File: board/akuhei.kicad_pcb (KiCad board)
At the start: 2 copper layers, 23 x 23.4 mm, 9 parts, among them J1 CLOCKPORT, J2 I2C, U2 PCA9564, U3 TLV70233DBV

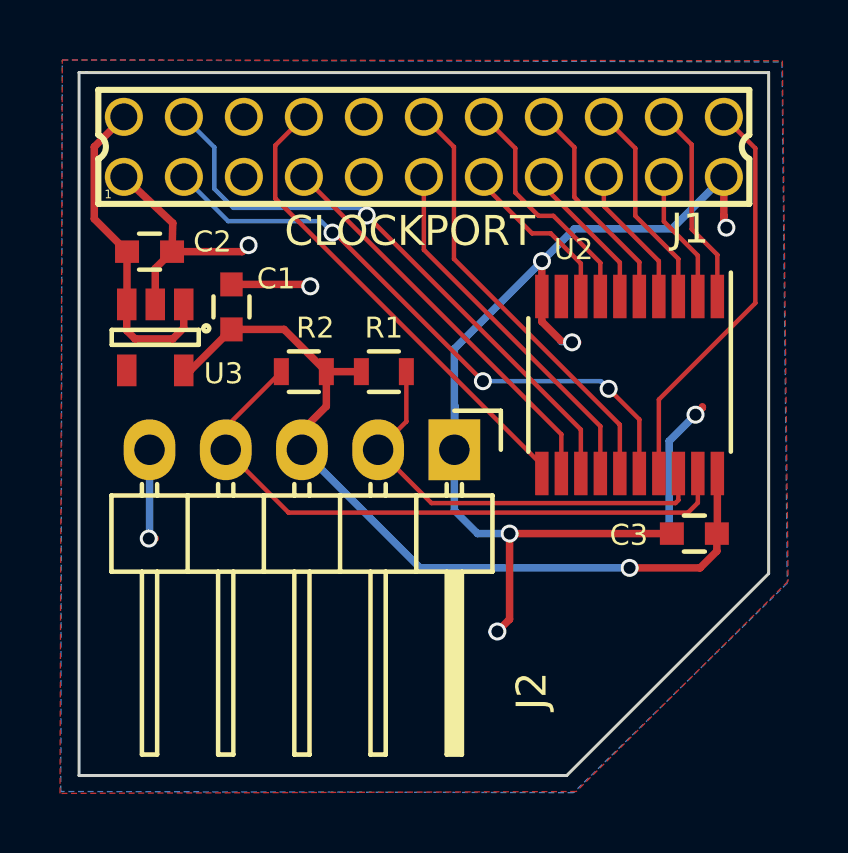
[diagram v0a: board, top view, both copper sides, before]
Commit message: removing error
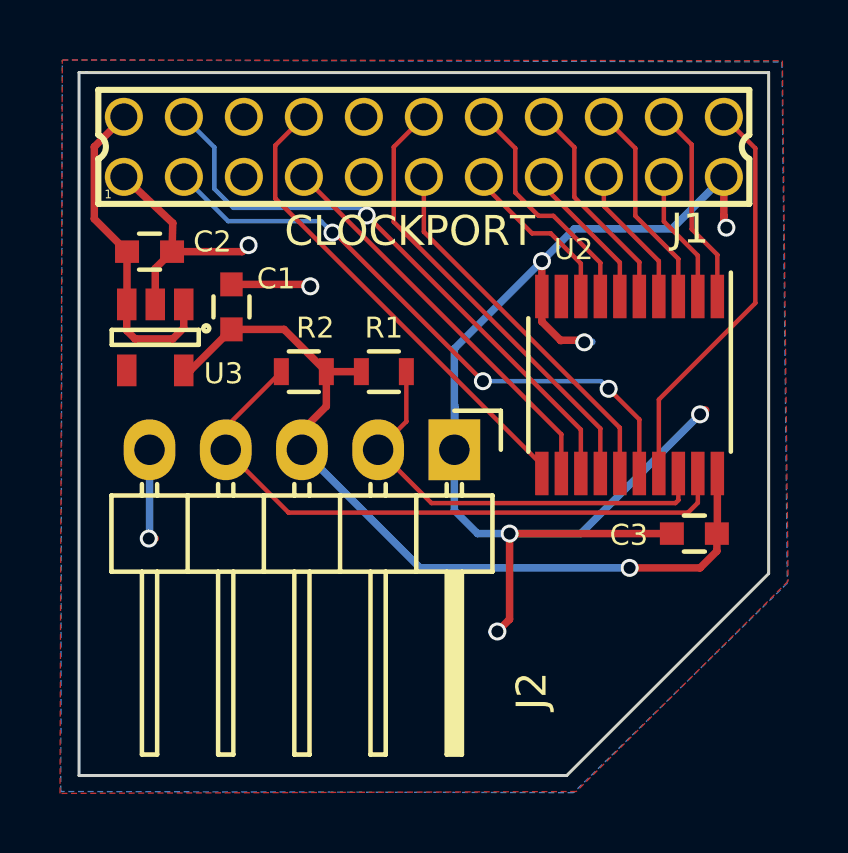
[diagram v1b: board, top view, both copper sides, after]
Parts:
- C1: value 1u -> 1uF
- C2: value u1 -> 0.1uF
- R1, R2: value 4k7 -> 4.7k
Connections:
- J1 pad 11: /A1 -> /A2
- J1 pad 12: /A2 -> /A1
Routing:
- net GND: track 48.9 -> 58.2 mm, vias 7 -> 9
- net (no net): track 5.22 -> 0.00 mm, vias 2 -> 0
- net /A1: track 12.3 -> 15.2 mm
- net /A2: track 14.6 -> 12.6 mm
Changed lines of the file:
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@@
     (links 36)
     (no_connects 0)
-    (area 132.3867 96.2279 160.286701 124.42)
+    (area 136.601999 96.596999 159.689001 120.128501)
     (thickness 1.6)
     (drawings 9)
-    (tracks 163)
+    (tracks 165)
     (zones 0)
     (modules 9)
@@
     (visible_elements 7FFFFFFF)
     (pcbplotparams
-      (layerselection 0x20020_00000000)
+      (layerselection 0x210f8_80000001)
       (usegerberextensions false)
       (excludeedgelayer true)
@@
       (viasonmask false)
       (mode 1)
-      (useauxorigin false)
+      (useauxorigin true)
       (hpglpennumber 1)
       (hpglpenspeed 20)
@@
       (effects (font (size 0.7 0.7) (thickness 0.15)))
     )
-    (fp_text value 1u (at -0.0381 0.0127 180) (layer F.Fab)
+    (fp_text value 1uF (at -0.0381 0.0127 180) (layer F.Fab)
       (effects (font (size 0.5 0.5) (thickness 0.125)))
     )
@@
       (effects (font (size 0.7 0.7) (thickness 0.15)))
     )
-    (fp_text value u1 (at 0.0254 -0.0508 90) (layer F.Fab)
+    (fp_text value 0.1uF (at 0.0254 -0.0508 90) (layer F.Fab)
       (effects (font (size 0.5 0.5) (thickness 0.125)))
     )
@@
       (net 11 "Net-(J1-Pad10)"))
     (pad 11 thru_hole circle (at 0 1) (size 1.27 1.27) (drill 0.9) (layers *.Cu *.Mask)
+      (net 13 /A2))
+    (pad 12 thru_hole circle (at 0 -1) (size 1.27 1.27) (drill 0.9) (layers *.Cu *.Mask)
       (net 12 /A1))
-    (pad 12 thru_hole circle (at 0 -1) (size 1.27 1.27) (drill 0.9) (layers *.Cu *.Mask)
-      (net 13 /A2))
     (pad 13 thru_hole circle (at 2 1) (size 1.27 1.27) (drill 0.9) (layers *.Cu *.Mask)
       (net 14 /D7))
@@
       (effects (font (size 0.7 0.7) (thickness 0.15)))
     )
-    (fp_text value 4k7 (at -0.0381 0 270) (layer F.Fab)
+    (fp_text value 4.7k (at -0.0381 0 270) (layer F.Fab)
       (effects (font (size 0.5 0.5) (thickness 0.125)))
     )
@@
       (effects (font (size 0.7 0.7) (thickness 0.15)))
     )
-    (fp_text value 4k7 (at 0.0254 -0.0254 90) (layer F.Fab)
+    (fp_text value 4.7k (at 0.0254 -0.0254 90) (layer F.Fab)
       (effects (font (size 0.5 0.5) (thickness 0.125)))
     )
@@
   (gr_line (start 159.639 96.647) (end 159.639 113.3475) (angle 90) (layer Edge.Cuts) (width 0.1))
   (gr_line (start 136.906 96.647) (end 159.639 96.647) (angle 90) (layer Edge.Cuts) (width 0.1))
-  (segment (start 156.3243 111.9759) (end 156.3243 108.9279) (width 0.25) (layer B.Cu) (net 0))
-  (segment (start 157.4292 107.823) (end 157.4292 107.7849) (width 0.25) (layer F.Cu) (net 0))
-  (segment (start 157.2006 108.0516) (end 157.4292 107.823) (width 0.25) (layer F.Cu) (net 0))
-  (via (at 157.2006 108.0516) (size 0.6) (drill 0.4) (layers F.Cu B.Cu) (net 0))
-  (segment (start 156.3243 108.9279) (end 157.2006 108.0516) (width 0.25) (layer B.Cu) (net 0))
-  (segment (start 152.7175 105.6132) (end 153.0604 105.6132) (width 0.25) (layer B.Cu) (net 0))
-  (segment (start 153.0858 105.6386) (end 153.2763 105.6386) (width 0.25) (layer F.Cu) (net 0))
-  (via (at 153.0858 105.6386) (size 0.6) (drill 0.4) (layers F.Cu B.Cu) (net 0))
-  (segment (start 153.0604 105.6132) (end 153.0858 105.6386) (width 0.25) (layer B.Cu) (net 0))
   (segment (start 144.0815 109.22) (end 148.0185 113.157) (width 0.25) (layer B.Cu) (net 1))
   (segment (start 157.9125 112.5975) (end 157.9125 112.014) (width 0.25) (layer F.Cu) (net 1))
@@
   (segment (start 140.142 106.5735) (end 140.366 106.5735) (width 0.25) (layer F.Cu) (net 1))
   (segment (start 140.366 106.5735) (end 141.732 105.2075) (width 0.25) (layer F.Cu) (net 1))
+  (segment (start 151.003 112.014) (end 153.3779 112.014) (width 0.25) (layer B.Cu) (net 2))
+  (segment (start 157.4927 107.8992) (end 157.5435 107.8992) (width 0.25) (layer F.Cu) (net 2))
+  (segment (start 157.353 108.0389) (end 157.4927 107.8992) (width 0.25) (layer F.Cu) (net 2))
+  (via (at 157.353 108.0389) (size 0.6) (drill 0.4) (layers F.Cu B.Cu) (net 2))
+  (segment (start 153.3779 112.014) (end 157.353 108.0389) (width 0.25) (layer B.Cu) (net 2))
+  (segment (start 152.69845 105.56875) (end 153.42235 105.56875) (width 0.25) (layer F.Cu) (net 2))
+  (segment (start 153.5049 105.6259) (end 153.7462 105.6259) (width 0.25) (layer B.Cu) (net 2))
+  (segment (start 153.4922 105.6386) (end 153.5049 105.6259) (width 0.25) (layer B.Cu) (net 2))
+  (via (at 153.4922 105.6386) (size 0.6) (drill 0.4) (layers F.Cu B.Cu) (net 2))
+  (segment (start 153.42235 105.56875) (end 153.4922 105.6386) (width 0.25) (layer F.Cu) (net 2))
   (segment (start 139.0015 109.22) (end 139.0015 112.1537) (width 0.25) (layer B.Cu) (net 2))
   (segment (start 138.9761 112.1791) (end 139.192 112.1791) (width 0.25) (layer F.Cu) (net 2))
@@
   (segment (start 158.1455 101.4146) (end 158.1531 101.4222) (width 0.25) (layer F.Cu) (net 2))
   (segment (start 152.0785 104.111) (end 152.0785 104.9488) (width 0.25) (layer F.Cu) (net 2))
-  (segment (start 152.0785 104.9488) (end 152.7175 105.5878) (width 0.25) (layer F.Cu) (net 2))
+  (segment (start 152.0785 104.9488) (end 152.69845 105.56875) (width 0.25) (layer F.Cu) (net 2))
+  (segment (start 152.69845 105.56875) (end 152.7175 105.5878) (width 0.25) (layer F.Cu) (net 2))
   (segment (start 149.1615 109.22) (end 149.1615 109.22) (width 0.25) (layer B.Cu) (net 2))
   (segment (start 149.1615 109.22) (end 149.1869 107.7595) (width 0.25) (layer B.Cu) (net 2))
@@
   (segment (start 143.1925 100.838) (end 143.1925 99.0765) (width 0.15) (layer F.Cu) (net 9))
   (segment (start 143.1925 99.0765) (end 144.1455 98.1235) (width 0.15) (layer F.Cu) (net 9))
-  (segment (start 154.0285 110.011) (end 154.0285 108.4355) (width 0.15) (layer F.Cu) (net 12))
-  (segment (start 148.1455 102.5525) (end 148.1455 100.1235) (width 0.15) (layer F.Cu) (net 12))
-  (segment (start 154.0285 108.4355) (end 148.1455 102.5525) (width 0.15) (layer F.Cu) (net 12))
-  (segment (start 154.6785 110.011) (end 154.6785 108.387) (width 0.15) (layer F.Cu) (net 13))
-  (segment (start 149.1488 99.1268) (end 148.1455 98.1235) (width 0.15) (layer F.Cu) (net 13))
-  (segment (start 149.1488 102.8573) (end 149.1488 99.1268) (width 0.15) (layer F.Cu) (net 13))
-  (segment (start 154.6785 108.387) (end 149.1488 102.8573) (width 0.15) (layer F.Cu) (net 13))
+  (segment (start 154.0285 110.011) (end 154.0285 108.5117) (width 0.15) (layer F.Cu) (net 12) (status 400000))
+  (segment (start 147.1422 99.1268) (end 148.1455 98.1235) (width 0.15) (layer F.Cu) (net 12) (status 800000))
+  (segment (start 147.1422 101.6254) (end 147.1422 99.1268) (width 0.15) (layer F.Cu) (net 12))
+  (segment (start 154.0285 108.5117) (end 147.1422 101.6254) (width 0.15) (layer F.Cu) (net 12))
+  (segment (start 154.6785 110.011) (end 154.6785 108.4886) (width 0.15) (layer F.Cu) (net 13) (status 400000))
+  (segment (start 148.1455 101.9556) (end 148.1455 100.1235) (width 0.15) (layer F.Cu) (net 13) (status 800000))
+  (segment (start 154.6785 108.4886) (end 148.1455 101.9556) (width 0.15) (layer F.Cu) (net 13))
   (segment (start 150.1455 100.1235) (end 150.1455 100.3996) (width 0.15) (layer F.Cu) (net 14))
   (segment (start 150.1455 100.3996) (end 151.7523 102.0064) (width 0.15) (layer F.Cu) (net 14))
